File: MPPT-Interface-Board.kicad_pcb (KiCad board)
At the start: 2 copper layers, 41.8 x 42.8 mm, 39 parts, among them J1 FIRST MPPT, J2 LAST MPPT, J3 CarCAN In, J4 CarCAN Out, J5 FUSEBOX, Q1 PMV35EPER, U1 RI3-1209S

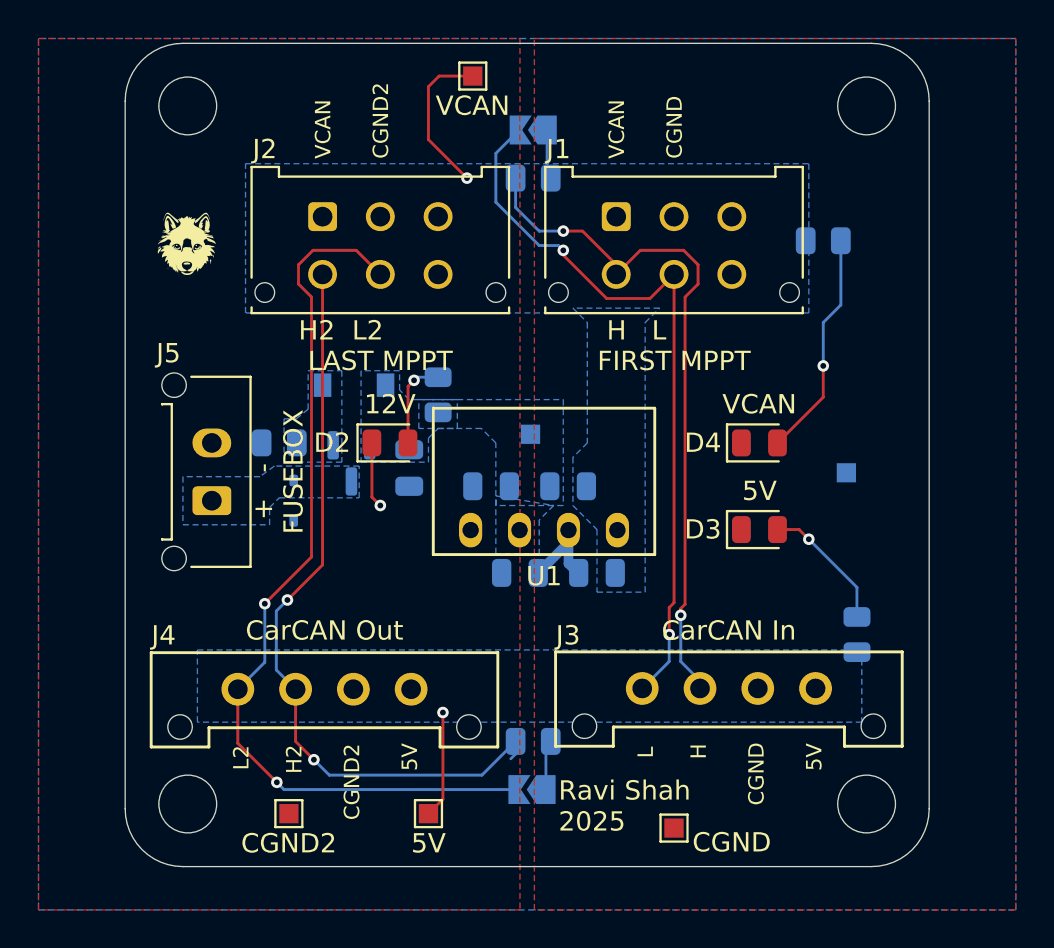
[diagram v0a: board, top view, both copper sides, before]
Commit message: Changed up to interface data acq leader
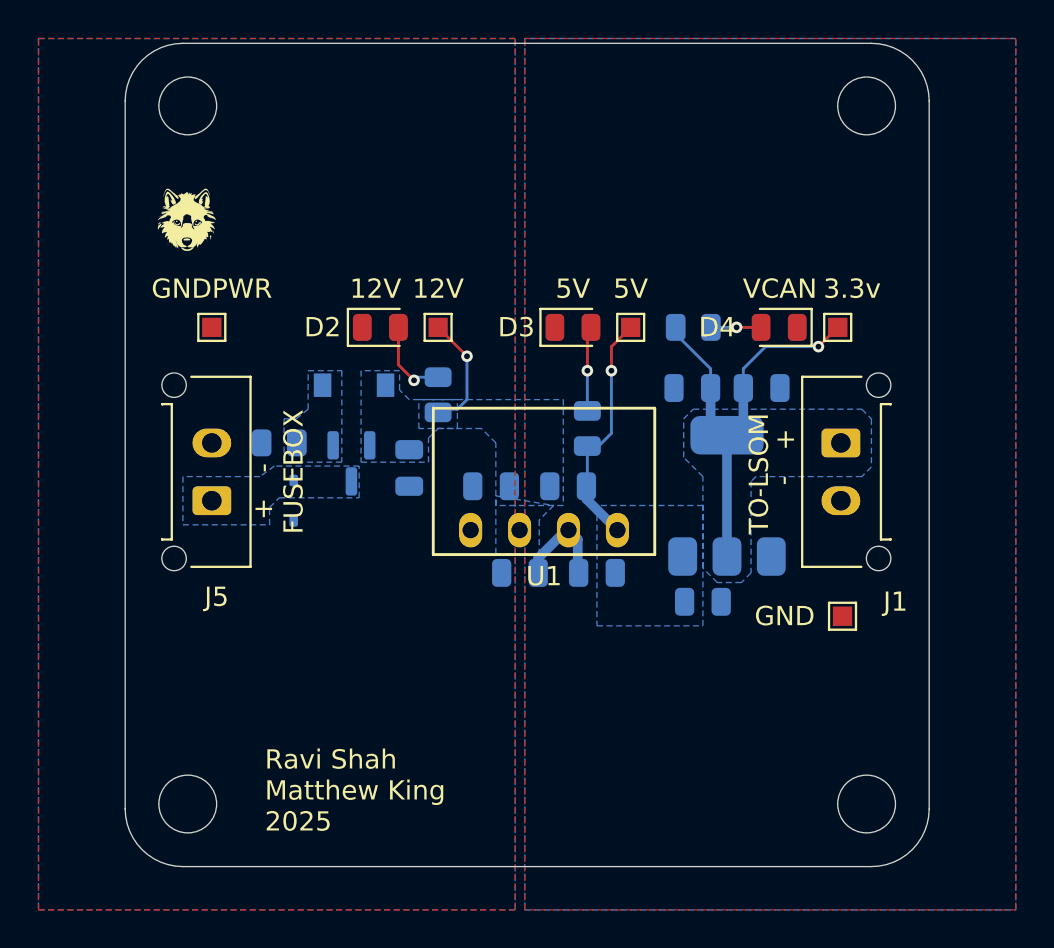
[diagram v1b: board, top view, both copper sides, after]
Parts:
- removed J2: LAST MPPT, Connector_Molex:Molex_Micro-Fit_3.0_43045-0612_2x03_P3.00mm_Vertical
- removed J3: CarCAN In, UTSVT-Connectors:Molex_MicroFit3.0_1x4xP3.00mm_PolarizingPeg_Vertical
- removed J4: CarCAN Out, UTSVT-Connectors:Molex_MicroFit3.0_1x4xP3.00mm_PolarizingPeg_Vertical
- removed JP1: CAN END, Jumper:SolderJumper-2_P1.3mm_Open_TrianglePad1.0x1.5mm
- removed JP2: CAN START, Jumper:SolderJumper-2_P1.3mm_Open_TrianglePad1.0x1.5mm
- removed LOGO1: UTSVT Logo, UTSVT-Special:UTSVT_Logo_Symbol
- removed R1, R6: 120, Resistor_SMD:R_0805_2012Metric
- removed TP6: CGND2, TestPoint:TestPoint_Pad_1.0x1.0mm
- added C6: 10uF, Capacitor_SMD:C_0805_2012Metric, B.Cu at (125.8, 91.5)
- added C7: 10uF, Capacitor_SMD:C_0805_2012Metric, B.Cu at (125.2, 80.4)
- added C8: 10uF, Capacitor_SMD:C_0805_2012Metric, B.Cu at (128.8, 80.4)
- added U2: NCP1117-3.3_SOT223, Package_TO_SOT_SMD:SOT-223-3_TabPin2, B.Cu at (127.0, 86.0)
- J1: value FIRST MPPT -> PWR-LSOM; footprint Connector_Molex:Molex_Micro-Fit_3.0_43045-0612_2x03_P3.00mm_Vertical -> Connector_Molex:Molex_Micro-Fit_3.0_43650-0215_1x02_P3.00mm_Vertical
- TP1: value CGND -> GND
- TP2, TP4: moved to F.Cu
- TP5: value VCAN -> 3.3v
- U1: value RI3-1209S -> RI3-1205S
- moved TP2 33.8 mm to (100.2, 77.2), turned to 0 degrees
- moved TP3 27.3 mm to (122.0, 77.2)
- moved TP5 23.0 mm to (132.8, 77.2)
- moved G*** 19.5 mm to (124.2, 101.5), turned to 0 degrees
- moved R4 17.6 mm to (119.8, 82.5)
- moved J1 16.6 mm to (132.9, 83.2), turned to -90 degrees
- moved D3 14.3 mm to (119.0, 77.2)
- moved TP1 14.1 mm to (133.0, 92.2)
- moved R5 8.11 mm to (125.2, 77.2)
- moved TP4 7.34 mm to (112.0, 77.2), turned to 0 degrees
- moved D4 6.09 mm to (129.7, 77.2), turned to 180 degrees
- moved D2 6.02 mm to (109.0, 77.2)
- moved G*** 1.25 mm to (99.0, 71.8)
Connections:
- C2 pad 1: V_CAN -> +5V
- C4 pad 2: V_CAN -> +5V
- J1 pad 1: V_CAN -> +3.3v
- R5 pad 1: V_CAN -> +3.3v
- TP5 pad 1: V_CAN -> +3.3v
- U1 pad 4: V_CAN -> +5V
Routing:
- net /CAN_L2: track 47.3 -> 0.00 mm, vias 2 -> 0
- net /CAN_H2: track 39.5 -> 0.00 mm, vias 2 -> 0
- net /CAN_L: track 38.4 -> 0.00 mm, vias 2 -> 0
- net /CAN_H: track 36.3 -> 0.00 mm, vias 2 -> 0
- net +3.3v: track 0.00 -> 22.6 mm, vias 0 -> 1
- net Net-(D4-A): track 11.9 -> 2.61 mm
- net V_CAN: track 8.11 -> 0.00 mm, vias 1 -> 0
- net +5V: track 5.56 -> 12.5 mm
- net +12V_PROT: track 0.00 -> 6.15 mm, vias 0 -> 1
- net GNDPWR: track 3.43 -> 0.00 mm, vias 1 -> 0
- net Net-(JP1-A): track 2.60 -> 0.00 mm
- net Net-(JP2-A): track 2.58 -> 0.00 mm
- net Net-(D3-A): track 6.91 -> 4.42 mm
- added copper zone on B.Cu, net +3.3v
- added copper zone on B.Cu, net CGND
- added copper zone on F.Cu, net GNDPWR
- removed copper zone on F.Cu, net CGND2
- removed copper zone on B.Cu, net V_CAN
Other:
- board text added: "Ravi Shah Matthew King 2025"
- board text added: "TO-LSOM"
- board text removed: "5V"
- board text removed: "CGND"
- board text removed: "CGND2"
- board text removed: "H"
- board text removed: "H L"
- board text removed: "H2"
- board text removed: "H2 L2"
- board text removed: "L"
- board text removed: "L2"
- board text removed: "Ravi Shah 2025"
- board text removed: "VCAN"

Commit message: Smaller version - gerbers made
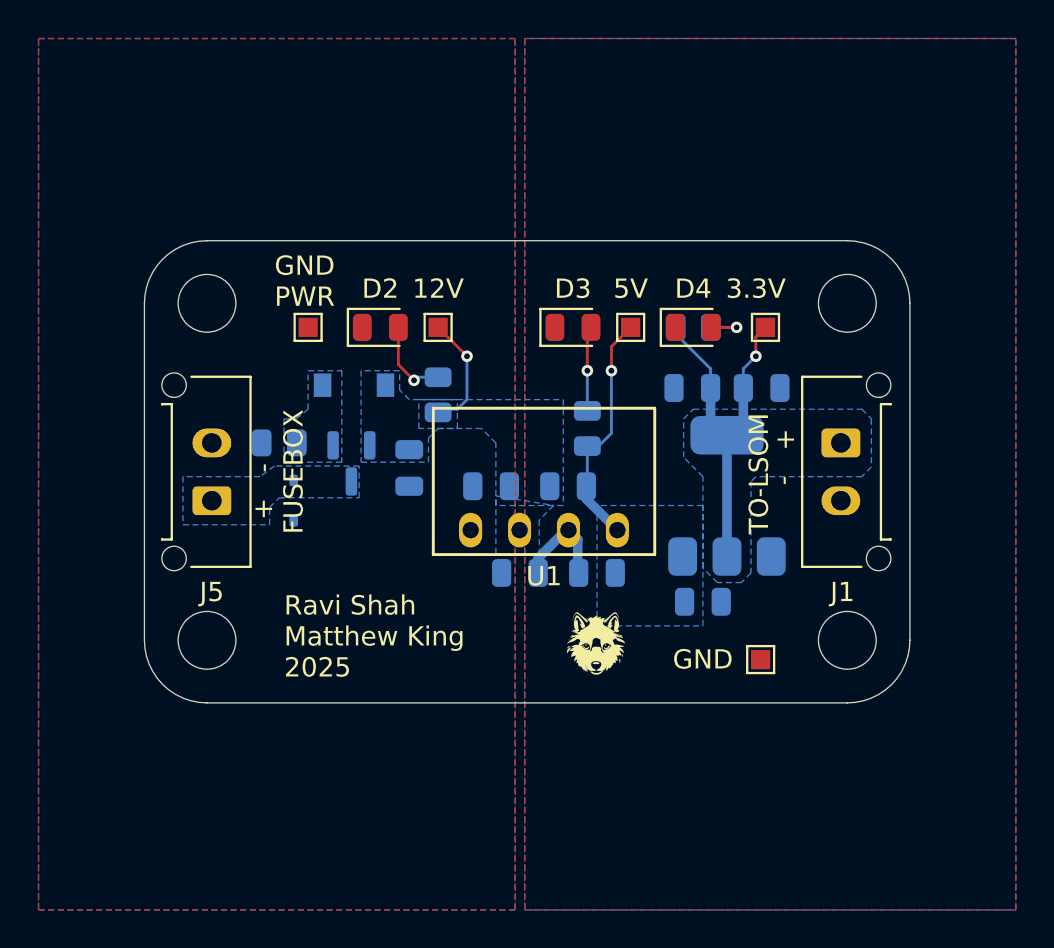
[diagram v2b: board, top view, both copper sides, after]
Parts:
- D4: value VCAN -> 3.3V
- G***: moved to B.Cu
- moved G*** 30.6 mm to (120.2, 93.8)
- moved G*** 27.9 mm to (116.5, 74.8), turned to 180 degrees
- moved G*** 19.7 mm to (109.0, 92.5)
- moved H1 10.3 mm to (100.0, 76.0)
- moved H2 10.3 mm to (133.2, 76.0)
- moved H3 8.56 mm to (133.2, 93.5)
- moved H4 8.56 mm to (100.0, 93.5)
- moved TP2 5.00 mm to (105.2, 77.2)
- moved TP1 4.81 mm to (128.8, 94.5)
- moved D4 4.46 mm to (125.2, 77.2), turned to 0 degrees
- moved TP5 3.75 mm to (129.0, 77.2)
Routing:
- net +3.3v: track 22.6 -> 19.4 mm
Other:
- board size 41.8 x 42.8 mm -> 39.8 x 24 mm
- board text added: "GND PWR"
